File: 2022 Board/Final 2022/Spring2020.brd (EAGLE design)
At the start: 63 x 65 mm, 21 parts, among them U1 TB67H401FTG(O,EL), U2 ABX00012

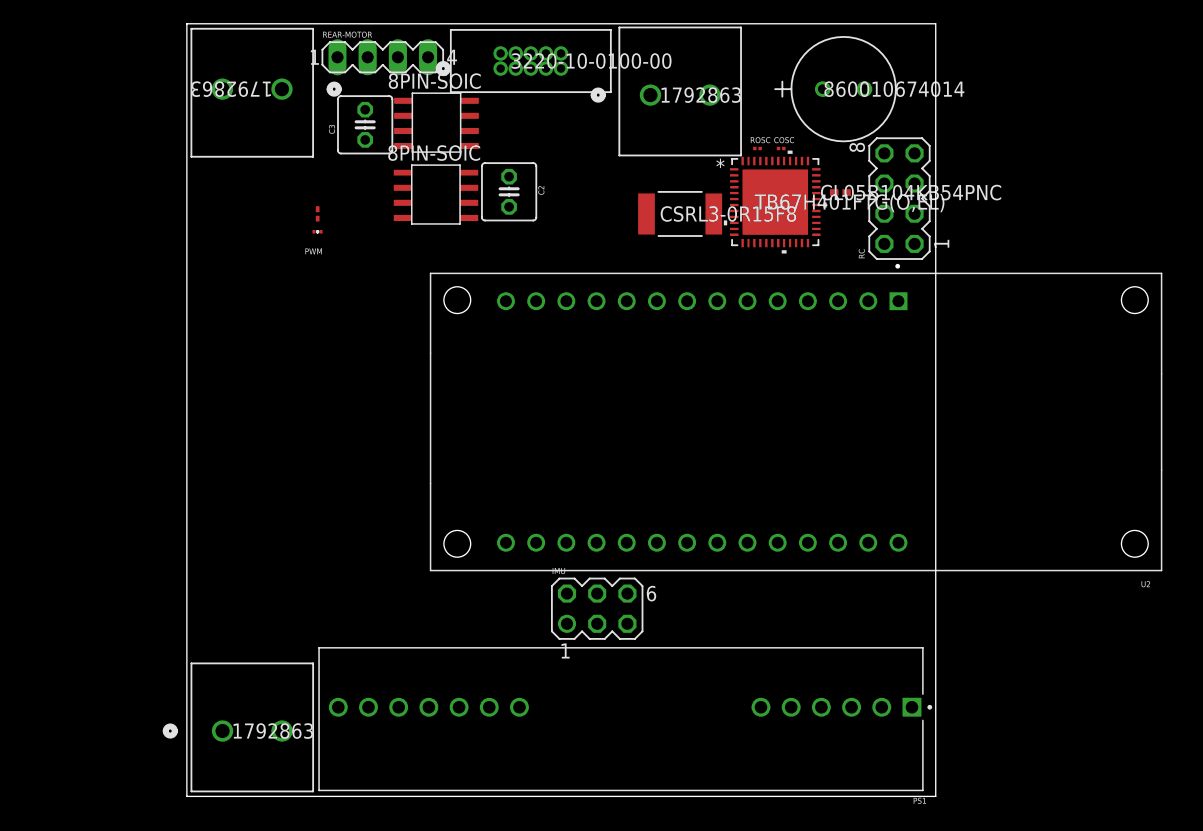
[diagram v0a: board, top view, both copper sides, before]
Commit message: Almost completely working board
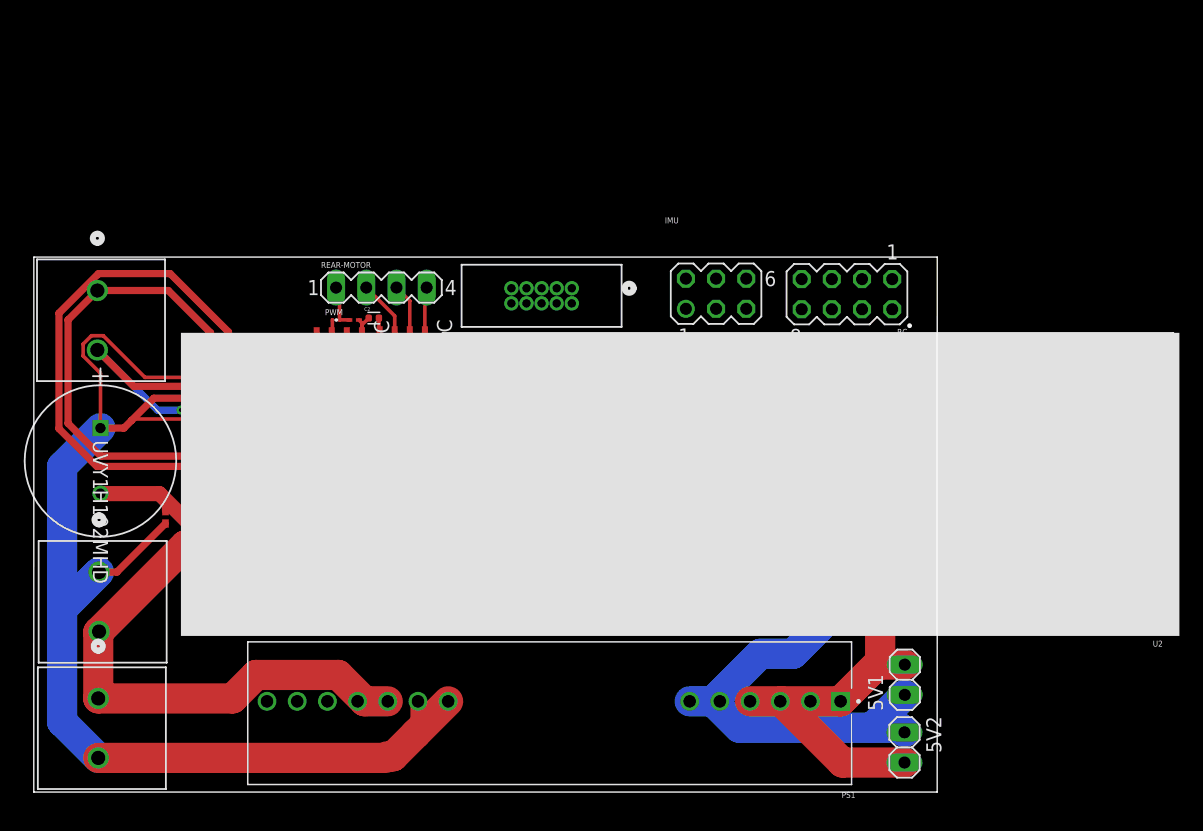
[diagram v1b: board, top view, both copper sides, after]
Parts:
- removed CVM1: 860010674014, Test:CAP_4014_WRE
- added 5V1, 5V2: (no value), pinhead:1X02
- added C1: CL05A105KP5NNNC, SnapEDA Library:CAPC1005X55N
- C2: value (none) -> CL05A105KP5NNNC; device resistor:C025-050X050 -> SnapEDA Library:CAPC1005X55N
- C3: value (none) -> UVY1H102MHD; device resistor:C025-050X050 -> Test2:CAP_12.5_X_25_NCH
- moved CVM2 63.0 mm to (16.2, 30.5), turned to 90 degrees
- moved FRT_MTR 49.3 mm to (10.5, 49.6), turned to 270 degrees
- moved U1 48.4 mm to (22.0, 40.5), turned to 270 degrees
- moved COSC 46.3 mm to (27.0, 40.0), turned to 270 degrees
- moved RRS 45.3 mm to (21.4, 31.5), turned to 90 degrees
- moved ROSC 43.7 mm to (27.0, 42.0), turned to 270 degrees
- moved REAR_PWR 43.4 mm to (10.6, 25.9), turned to 270 degrees
- moved C3 33.9 mm to (10.7, 38.0), turned to 270 degrees
- moved IMU 28.3 mm to (62.5, 49.3)
- moved U$2 21.1 mm to (36.5, 43.0), turned to 90 degrees
- moved FRT_ENCODE 19.4 mm to (50.4, 49.7), turned to 180 degrees
- moved REAR-MOTOR 19.4 mm to (34.4, 49.8)
- moved U$7 16.9 mm to (31.2, 42.9), turned to 90 degrees
- moved C2 15.6 mm to (33.7, 47.2), turned to 0 degrees
- moved PWR_IN 10.8 mm to (10.5, 15.2), turned to 270 degrees
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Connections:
- removed net N$10: FRT_ENCODE.8
- removed net N$4: FRT_ENCODE.4
- removed net N$6: U2.20
- removed net N$7: U2.21
- new net FLMT: FRT_ENCODE.4, U2.7
- new net RLMT: FRT_ENCODE.8, U2.8
- net 3.3V: now also C1.1; no longer C2.1
- net 5V: now also 5V1.2, 5V2.2, C2.2; no longer C3.1
- net BKPWR: now also C3.2, PWR_IN.1, REAR_PWR.2; no longer CVM1.2, PWR_IN.2, REAR_PWR.1
- net F+: now also FRT_MTR.1; no longer FRT_MTR.2
- net F-: now also FRT_MTR.2; no longer FRT_MTR.1
- net FRT_PWM: now also U2.14
- net GND: now also 5V1.1, 5V2.1, C1.2, C2.1, C3.1, PWR_IN.2, REAR-MOTOR.4, REAR_PWR.1; no longer C2.2, C3.2, CVM1.1, PWR_IN.1, REAR-MOTOR.1, REAR_PWR.2
- net IMU-CS: now also IMU.4, U2.20; no longer IMU.2, U2.16
- net I_1: now also U2.13
- net I_2: now also U2.12
- net QUAD-A: now also U2.16
- net QUAD-B: now also U2.15
- net REAR-PWM: now also U2.9; no longer U2.12
- net REAR-PWMOUT: now also REAR-MOTOR.1; no longer REAR-MOTOR.2
- net REAR-TIMER: now also REAR-MOTOR.3; no longer REAR-MOTOR.4
- net REAR-TIMER-IN: now also U2.21
- net REVERSE: now also REAR-MOTOR.2; no longer REAR-MOTOR.3
- net SCK: now also IMU.2; no longer IMU.4
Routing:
- net GND: track 0.00 -> 184.3 mm
- net BKPWR: track 0.00 -> 75.2 mm
- net 5V: track 0.00 -> 60.2 mm
- net RS: track 0.00 -> 49.9 mm
- net F+: track 0.00 -> 41.3 mm
- net F-: track 0.00 -> 22.0 mm, vias 0 -> 1
- net 3.3V: track 0.00 -> 8.69 mm
- net REVERSE: track 0.00 -> 5.00 mm
- net REAR-TIMER: track 0.00 -> 4.48 mm
- net REAR-PWMOUT: track 0.00 -> 3.68 mm
- net REAR-PWM-5V: track 0.00 -> 1.39 mm
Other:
- board size 63 x 65 mm -> 76 x 45 mm
